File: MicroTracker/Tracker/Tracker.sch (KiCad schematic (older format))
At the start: 4 parts

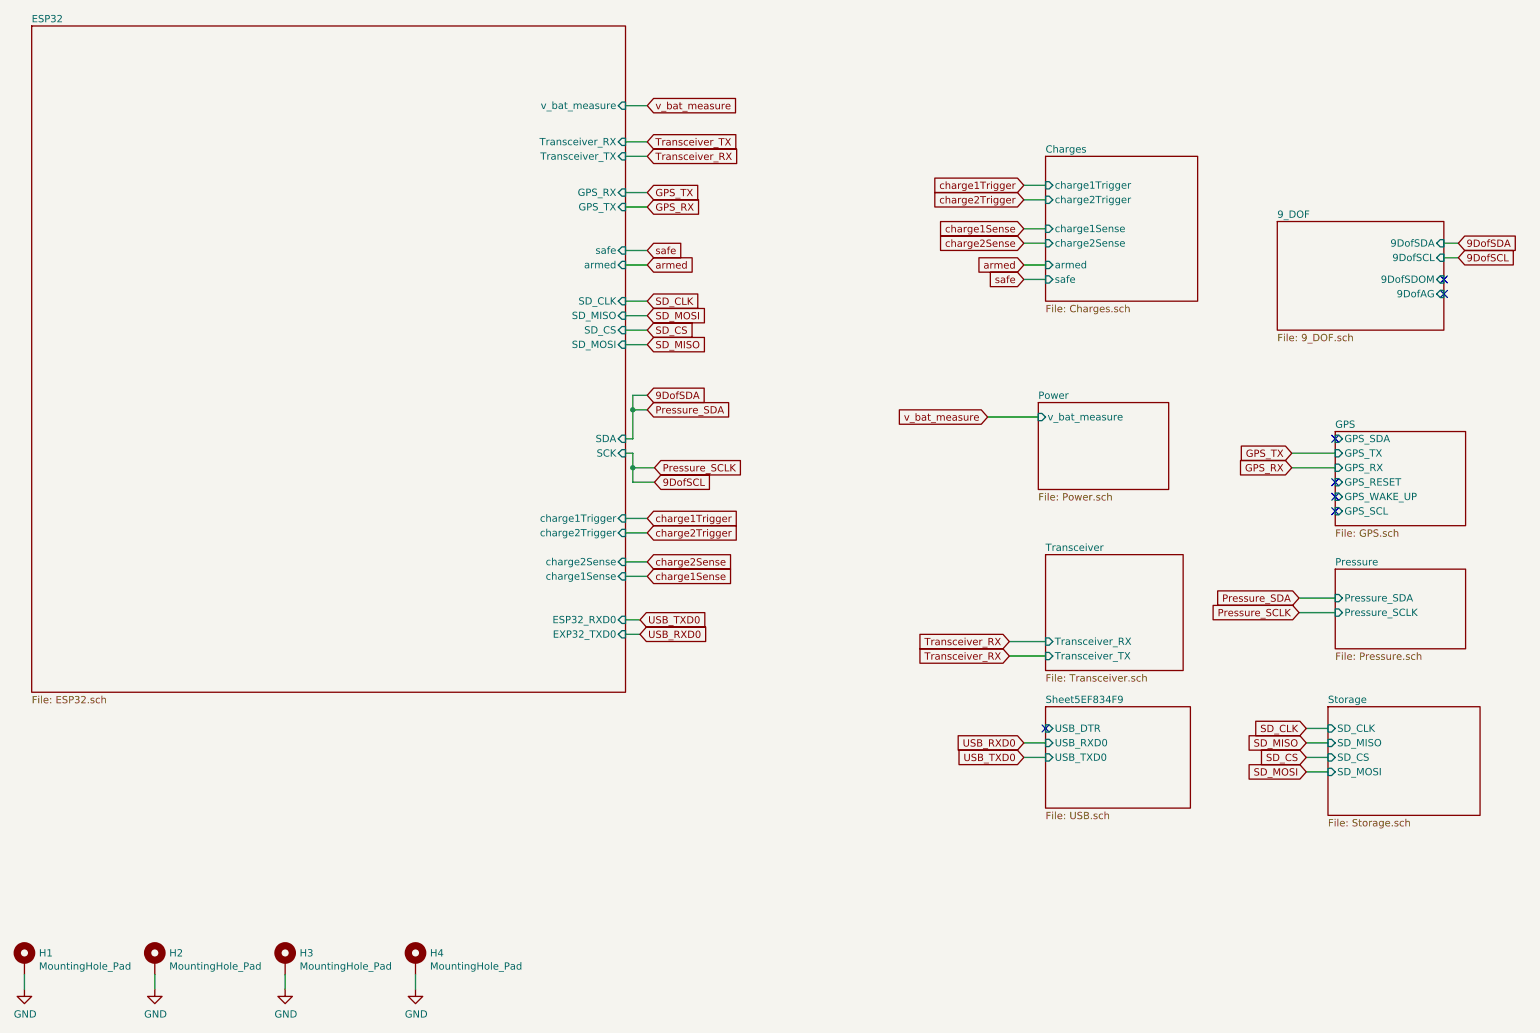
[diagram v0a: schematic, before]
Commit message: fixed errors
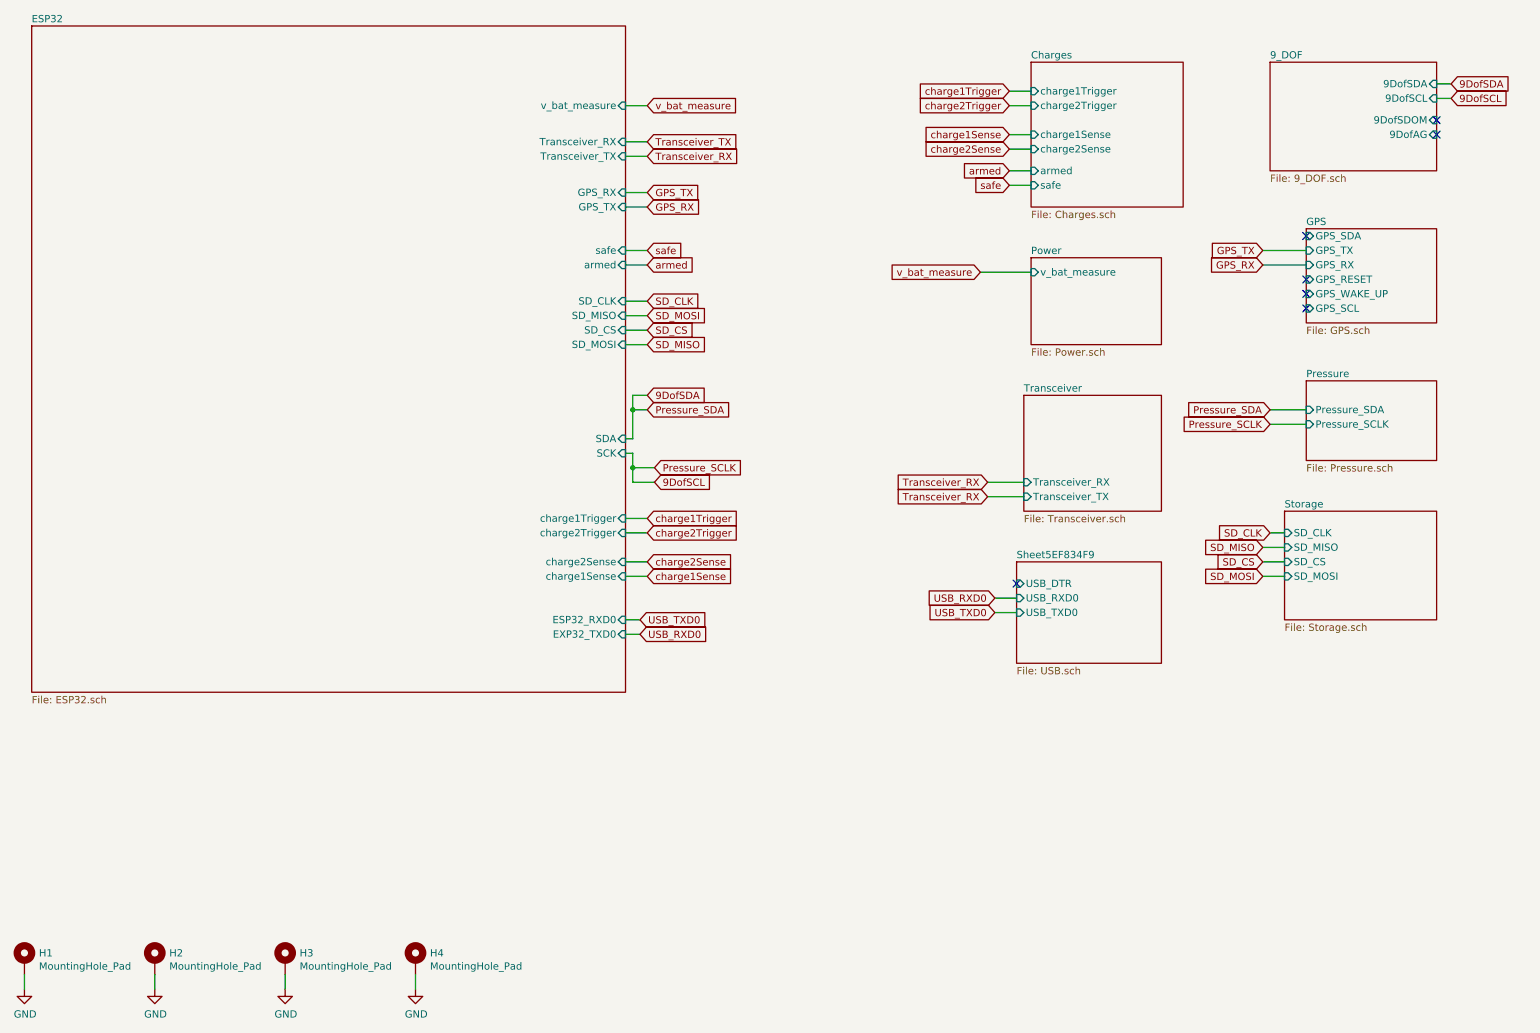
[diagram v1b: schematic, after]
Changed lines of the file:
@@
 $EndDescr
 $Sheet
-S 7800 3450 900  600
+S 7750 2450 900  600
 U 5EF7F21E
 F0 "Power" 50
 F1 "Power.sch" 50
-F2 "v_bat_measure" I L 7800 3550 50
-$EndSheet
-$Sheet
-S 9850 3650 900  650
+F2 "v_bat_measure" I L 7750 2550 50
+$EndSheet
+$Sheet
+S 9650 2250 900  650
 U 5EF7F258
 F0 "GPS" 50
 F1 "GPS.sch" 50
-F2 "GPS_TX" I L 9850 3800 50
-F3 "GPS_RX" I L 9850 3900 50
-F4 "GPS_RESET" I L 9850 4000 50
-F5 "GPS_WAKE_UP" I L 9850 4100 50
-F6 "GPS_SCL" I L 9850 4200 50
-F7 "GPS_SDA" I L 9850 3700 50
-$EndSheet
-$Sheet
-S 9850 4600 900  550
+F2 "GPS_TX" I L 9650 2400 50
+F3 "GPS_RX" I L 9650 2500 50
+F4 "GPS_RESET" I L 9650 2600 50
+F5 "GPS_WAKE_UP" I L 9650 2700 50
+F6 "GPS_SCL" I L 9650 2800 50
+F7 "GPS_SDA" I L 9650 2300 50
+$EndSheet
+$Sheet
+S 9650 3300 900  550
 U 5EF7F2B3
 F0 "Pressure" 50
 F1 "Pressure.sch" 50
-F2 "Pressure_SDA" I L 9850 4800 50
-F3 "Pressure_SCLK" I L 9850 4900 50
-$EndSheet
-$Sheet
-S 7850 4500 950  800
+F2 "Pressure_SDA" I L 9650 3500 50
+F3 "Pressure_SCLK" I L 9650 3600 50
+$EndSheet
+$Sheet
+S 7700 3400 950  800
 U 5EF7F30A
 F0 "Transceiver" 50
 F1 "Transceiver.sch" 50
-F2 "Transceiver_TX" I L 7850 5200 50
-F3 "Transceiver_RX" I L 7850 5100 50
+F2 "Transceiver_TX" I L 7700 4100 50
+F3 "Transceiver_RX" I L 7700 4000 50
 $EndSheet
 $Sheet
@@
 $EndSheet
 $Sheet
-S 7850 5550 1000 700
+S 7650 4550 1000 700
 U 5EF834FA
 F0 "Sheet5EF834F9" 50
 F1 "USB.sch" 50
-F2 "USB_DTR" I L 7850 5700 50
-F3 "USB_RXD0" I L 7850 5800 50
-F4 "USB_TXD0" I L 7850 5900 50
-$EndSheet
-Text GLabel 9600 4800 0    50   Input ~ 0
+F2 "USB_DTR" I L 7650 4700 50
+F3 "USB_RXD0" I L 7650 4800 50
+F4 "USB_TXD0" I L 7650 4900 50
+$EndSheet
+Text GLabel 9400 3500 0    50   Input ~ 0
 Pressure_SDA
-Text GLabel 9600 4900 0    50   Input ~ 0
+Text GLabel 9400 3600 0    50   Input ~ 0
 Pressure_SCLK
-Text GLabel 9550 3800 0    50   Input ~ 0
+Text GLabel 9350 2400 0    50   Input ~ 0
 GPS_TX
-Text GLabel 9550 3900 0    50   Input ~ 0
+Text GLabel 9350 2500 0    50   Input ~ 0
 GPS_RX
 Wire Wire Line
-	9550 3800 9850 3800
-Wire Wire Line
-	9550 3900 9850 3900
-Text GLabel 7450 3550 0    50   Input ~ 0
+	9350 2400 9650 2400
+Wire Wire Line
+	9350 2500 9650 2500
+Text GLabel 7400 2550 0    50   Input ~ 0
 v_bat_measure
 Wire Wire Line
-	7450 3550 7800 3550
-Wire Wire Line
-	9600 4800 9850 4800
-Wire Wire Line
-	9600 4900 9850 4900
+	7400 2550 7750 2550
+Wire Wire Line
+	9400 3500 9650 3500
+Wire Wire Line
+	9400 3600 9650 3600
 Text GLabel 5100 3500 2    50   Input ~ 0
 Pressure_SDA
@@
 v_bat_measure
 $Sheet
-S 9800 5550 1050 750
+S 9500 4200 1050 750
 U 5EF91B46
 F0 "Storage" 50
 F1 "Storage.sch" 50
-F2 "SD_CLK" I L 9800 5700 50
-F3 "SD_MISO" I L 9800 5800 50
-F4 "SD_CS" I L 9800 5900 50
-F5 "SD_MOSI" I L 9800 6000 50
-$EndSheet
-Text GLabel 7700 5800 0    50   Input ~ 0
+F2 "SD_CLK" I L 9500 4350 50
+F3 "SD_MISO" I L 9500 4450 50
+F4 "SD_CS" I L 9500 4550 50
+F5 "SD_MOSI" I L 9500 4650 50
+$EndSheet
+Text GLabel 7500 4800 0    50   Input ~ 0
 USB_RXD0
-Text GLabel 7700 5900 0    50   Input ~ 0
+Text GLabel 7500 4900 0    50   Input ~ 0
 USB_TXD0
 Text GLabel 5050 5050 2    50   Input ~ 0
@@
 USB_TXD0
 Wire Wire Line
-	7700 5800 7850 5800
-Wire Wire Line
-	7700 5900 7850 5900
+	7500 4800 7650 4800
+Wire Wire Line
+	7500 4900 7650 4900
 Wire Wire Line
 	5050 4950 4950 4950
 Wire Wire Line
 	4950 5050 5050 5050
-Text GLabel 7600 5100 0    50   Input ~ 0
+Text GLabel 7450 4000 0    50   Input ~ 0
 Transceiver_RX
-Text GLabel 7600 5200 0    50   Input ~ 0
+Text GLabel 7450 4100 0    50   Input ~ 0
 Transceiver_RX
 Wire Wire Line
-	7600 5100 7850 5100
-Wire Wire Line
-	7600 5200 7850 5200
+	7450 4000 7700 4000
+Wire Wire Line
+	7450 4100 7700 4100
 Text GLabel 5100 1750 2    50   Input ~ 0
 Transceiver_RX
@@
 Transceiver_TX
 $Sheet
-S 7850 1750 1050 1000
+S 7750 1100 1050 1000
 U 5EFA735D
 F0 "Charges" 50
 F1 "Charges.sch" 50
-F2 "charge1Trigger" I L 7850 1950 50
-F3 "charge2Trigger" I L 7850 2050 50
-F4 "charge2Sense" I L 7850 2350 50
-F5 "charge1Sense" I L 7850 2250 50
-F6 "armed" I L 7850 2500 50
-F7 "safe" I L 7850 2600 50
+F2 "charge1Trigger" I L 7750 1300 50
+F3 "charge2Trigger" I L 7750 1400 50
+F4 "charge2Sense" I L 7750 1700 50
+F5 "charge1Sense" I L 7750 1600 50
+F6 "armed" I L 7750 1850 50
+F7 "safe" I L 7750 1950 50
 $EndSheet
 Wire Wire Line
@@
 	4950 2100 5100 2100
 $Sheet
-S 9450 2200 1150 750
+S 9400 1100 1150 750
 U 5F07F54B
 F0 "9_DOF" 50
 F1 "9_DOF.sch" 50
-F2 "9DofSDA" I R 10600 2350 50
-F3 "9DofSCL" I R 10600 2450 50
-F4 "9DofSDOM" I R 10600 2600 50
-F5 "9DofAG" I R 10600 2700 50
-$EndSheet
-Text GLabel 10700 2350 2    50   Input ~ 0
+F2 "9DofSDA" I R 10550 1250 50
+F3 "9DofSCL" I R 10550 1350 50
+F4 "9DofSDOM" I R 10550 1500 50
+F5 "9DofAG" I R 10550 1600 50
+$EndSheet
+Text GLabel 10650 1250 2    50   Input ~ 0
 9DofSDA
-Text GLabel 10700 2450 2    50   Input ~ 0
+Text GLabel 10650 1350 2    50   Input ~ 0
 9DofSCL
 Text GLabel 5100 3400 2    50   Input ~ 0
@@
 Wire Wire Line
 	5000 3900 5000 4000
-Text GLabel 9650 5700 0    50   Input ~ 0
+Text GLabel 9400 4350 0    50   Input ~ 0
 SD_CLK
-Text GLabel 9650 5800 0    50   Input ~ 0
+Text GLabel 9350 4450 0    50   Input ~ 0
 SD_MISO
-Text GLabel 9650 5900 0    50   Input ~ 0
+Text GLabel 9350 4550 0    50   Input ~ 0
 SD_CS
-Text GLabel 9650 6000 0    50   Input ~ 0
+Text GLabel 9350 4650 0    50   Input ~ 0
 SD_MOSI
 Wire Wire Line
-	9650 5700 9800 5700
-Wire Wire Line
-	9650 5800 9800 5800
-Wire Wire Line
-	9650 5900 9800 5900
-Wire Wire Line
-	9650 6000 9800 6000
+	9350 4450 9500 4450
+Wire Wire Line
+	9350 4550 9500 4550
+Wire Wire Line
+	9350 4650 9500 4650
 Text GLabel 5100 2750 2    50   Input ~ 0
 SD_CLK
@@
 	4950 3050 5100 3050
 Wire Wire Line
-	10600 2350 10700 2350
-Wire Wire Line
-	10600 2450 10700 2450
+	10550 1250 10650 1250
+Wire Wire Line
+	10550 1350 10650 1350
 $Comp
 L Mechanical:MountingHole_Pad H1
@@
 Wire Wire Line
 	4950 4650 5100 4650
-Text GLabel 7700 1950 0    50   Input ~ 0
+Text GLabel 7600 1300 0    50   Input ~ 0
 charge1Trigger
-Text GLabel 7700 2050 0    50   Input ~ 0
+Text GLabel 7600 1400 0    50   Input ~ 0
 charge2Trigger
-Text GLabel 7700 2350 0    50   Input ~ 0
+Text GLabel 7600 1700 0    50   Input ~ 0
 charge2Sense
-Text GLabel 7700 2250 0    50   Input ~ 0
+Text GLabel 7600 1600 0    50   Input ~ 0
 charge1Sense
 Wire Wire Line
-	7700 1950 7850 1950
-Wire Wire Line
-	7700 2050 7850 2050
-Wire Wire Line
-	7700 2250 7850 2250
-Wire Wire Line
-	7700 2350 7850 2350
-NoConn ~ 9850 3700
-NoConn ~ 9850 4000
-NoConn ~ 9850 4100
-NoConn ~ 9850 4200
-NoConn ~ 7850 5700
+	7600 1300 7750 1300
+Wire Wire Line
+	7600 1400 7750 1400
+Wire Wire Line
+	7600 1600 7750 1600
+Wire Wire Line
+	7600 1700 7750 1700
+NoConn ~ 9650 2300
+NoConn ~ 9650 2600
+NoConn ~ 9650 2700
+NoConn ~ 9650 2800
+NoConn ~ 7650 4700
 Wire Wire Line
 	4950 1650 5100 1650
-Text GLabel 7700 2500 0    50   Input ~ 0
+Text GLabel 7600 1850 0    50   Input ~ 0
 armed
-Text GLabel 7700 2600 0    50   Input ~ 0
+Text GLabel 7600 1950 0    50   Input ~ 0
 safe
 Wire Wire Line
-	7700 2500 7850 2500
-Wire Wire Line
-	7700 2600 7850 2600
+	7600 1850 7750 1850
+Wire Wire Line
+	7600 1950 7750 1950
 Text GLabel 5100 2500 2    50   Input ~ 0
 armed
@@
 Wire Wire Line
 	4950 2500 5100 2500
-NoConn ~ 10600 2600
-NoConn ~ 10600 2700
+NoConn ~ 10550 1500
+NoConn ~ 10550 1600
+Wire Wire Line
+	9400 4350 9500 4350
 $EndSCHEMATC
